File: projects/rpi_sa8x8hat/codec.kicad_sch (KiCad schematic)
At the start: 24 parts, among them U4 TLV320AIC3204

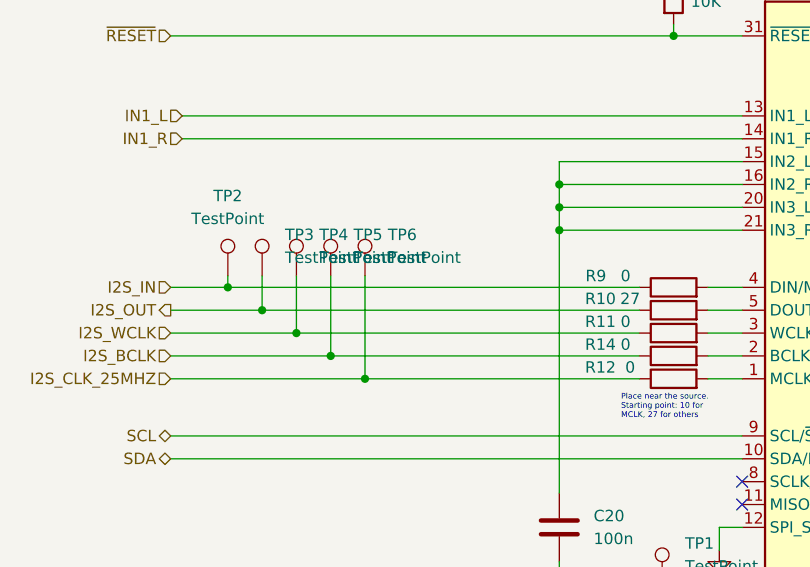
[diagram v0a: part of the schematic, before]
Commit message: WIP.
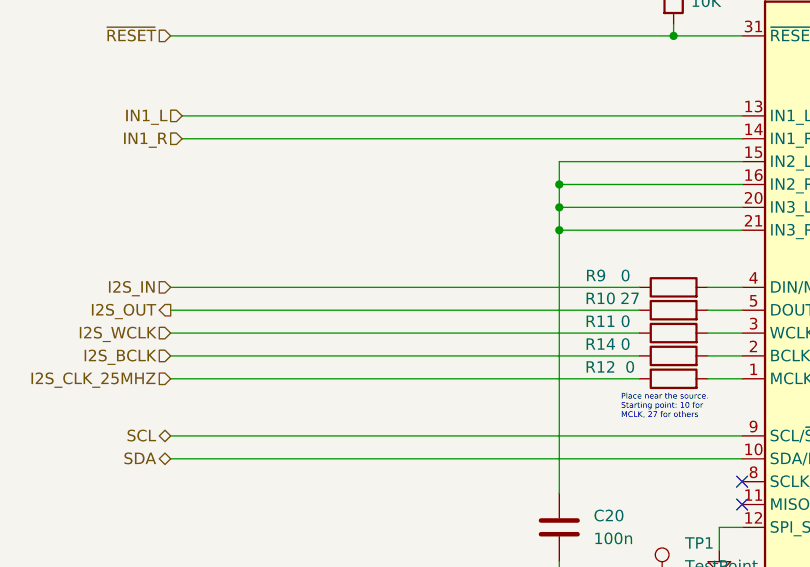
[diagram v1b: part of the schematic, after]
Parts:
- removed TP2, TP3, TP4, TP5, TP6: TestPoint, symbol Connector:TestPoint
- C10, C11, C15, C6, C8: footprint (none) -> Capacitor_SMD:C_0201_0603Metric
- C14, C20, C4, C5, C7, C9: footprint (none) -> Capacitor_SMD:C_0402_1005Metric
- R10, R11, R12, R14, R8, R9: footprint (none) -> Resistor_SMD:R_0402_1005Metric
- TP1: footprint (none) -> TestPoint:TestPoint_Pad_2.0x2.0mm
